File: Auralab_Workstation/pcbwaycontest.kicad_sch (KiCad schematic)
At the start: 12 parts, among them J1 Conn_Coaxial, Q1 BS170, SW1 SW_SPDT, U1 TL072, U2 MCP3201, U3 REF3033, U4 INA226

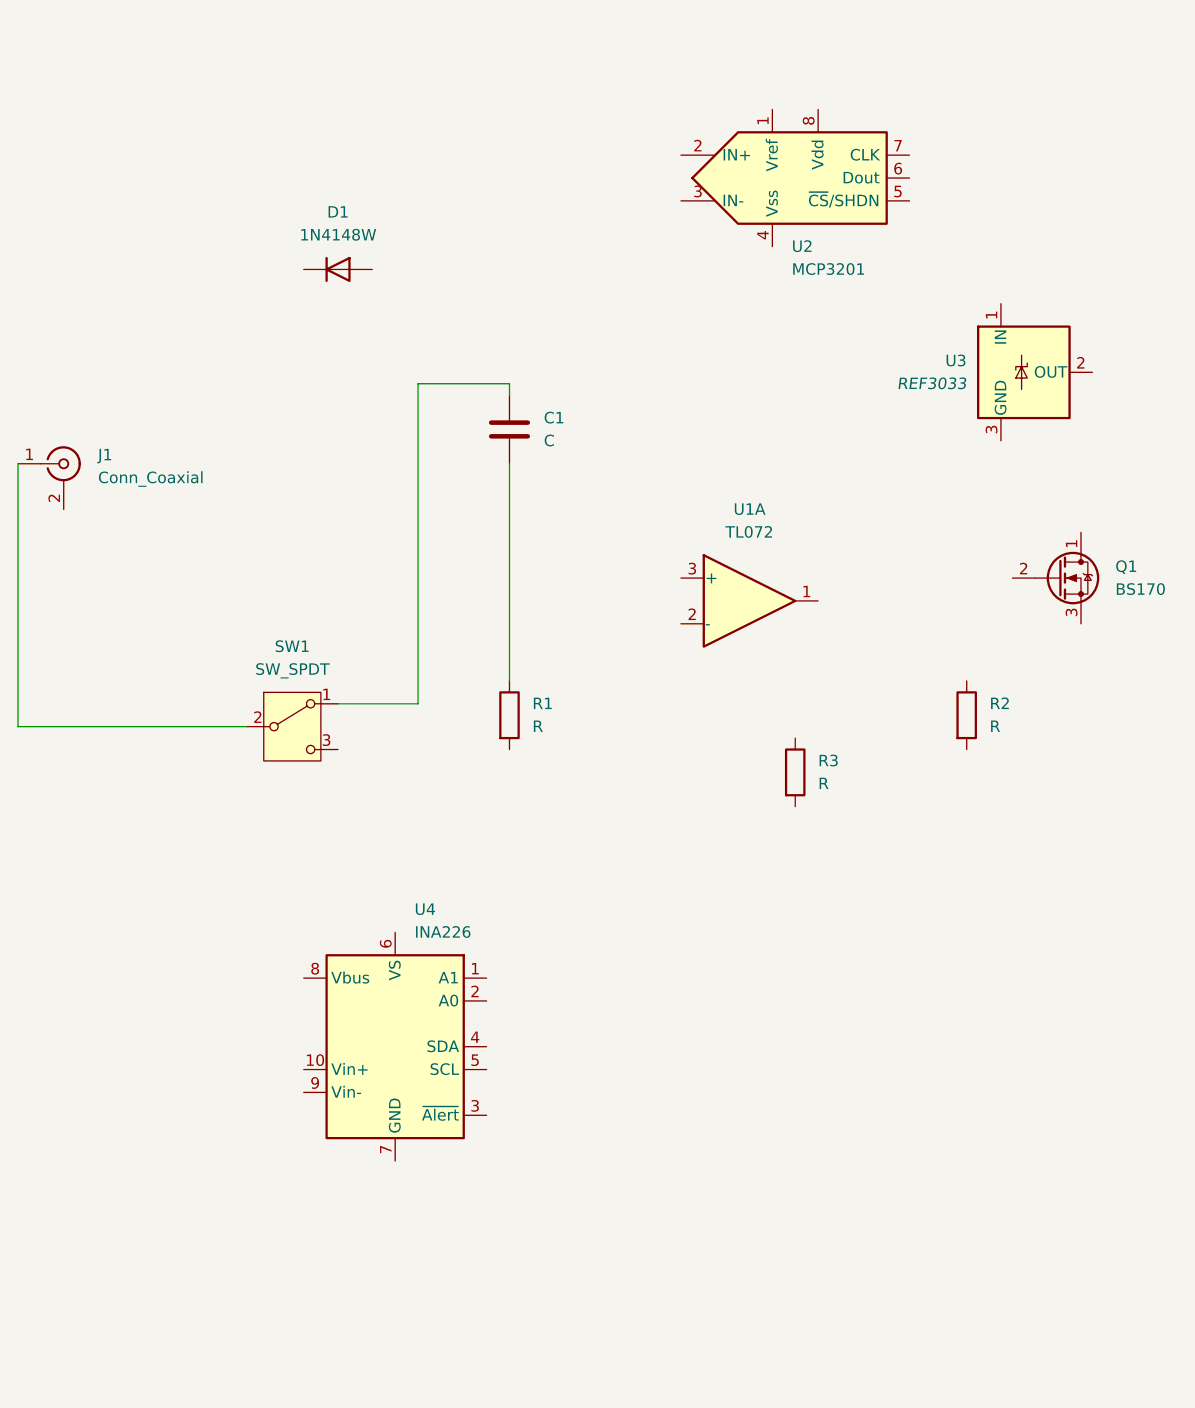
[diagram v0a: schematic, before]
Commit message: Add files via upload
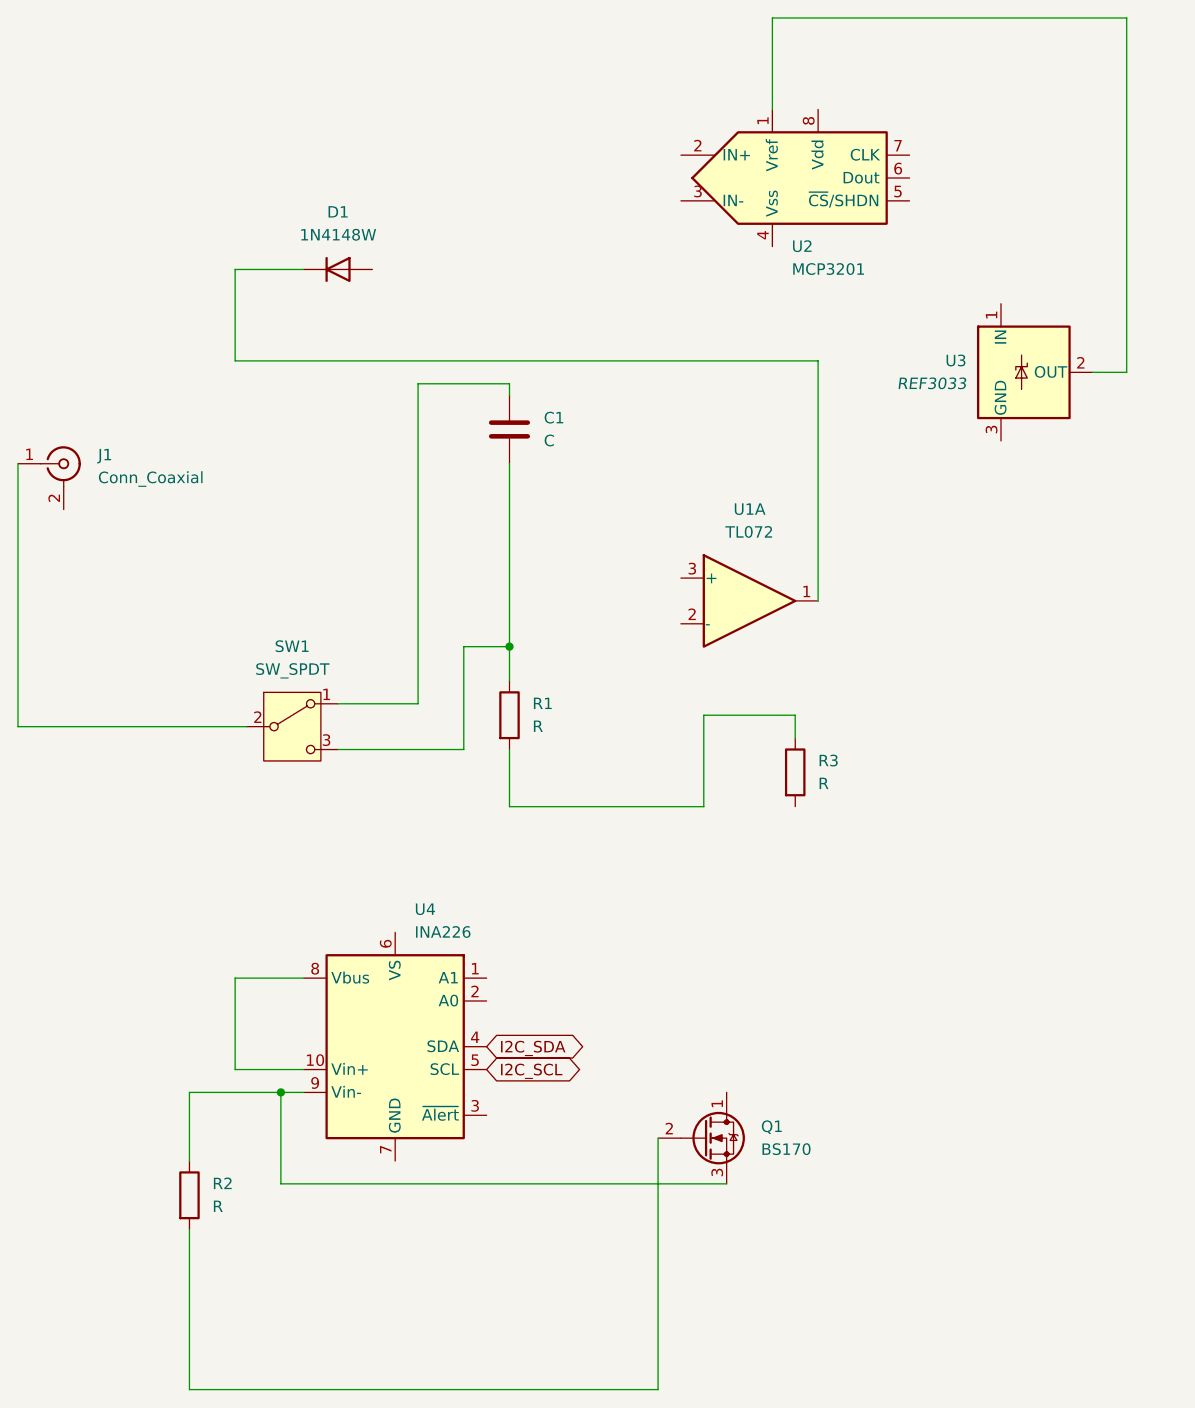
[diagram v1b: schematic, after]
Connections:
- net at U3.2 (OUT): now also U2.1 (Vref)
- net at U1.1: now also D1.1 (K)
- net at SW1.3 (C): now also C1.2, R1.1
- net at R2.1: now also Q1.3 (S), U4.9 (Vin-)
- net at R2.2: now also Q1.2 (G)
- net at R3.1: now also R1.2
- net at U4.10 (Vin+): now also U4.8 (Vbus)
- net I2C_SDA: now reaches U4.4 (SDA)
- net I2C_SCL: now reaches U4.5 (SCL)
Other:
- moved on the sheet: Q1, R2
